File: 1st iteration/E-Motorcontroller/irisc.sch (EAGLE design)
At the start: 173 parts, among them IC1 L298, IC2 L298, U1 KXTJ3-1057, U11 LTC6655CHMS8-3.3PBF, U4 PCA9685, U5 ANALOG_DEVICES_ADXRS646BBGZAN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, U6 ANALOG_DEVICES_AD7997BRUZ-1RE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, U7 MELEXIS_TECHNOLOGIES_MLX90393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, U8 ANALOG_DEVICES_AD7997BRUZ-1RE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, X1 RASPI_BOARD_B+_E4, Y1 16MHz

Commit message: Removed unnecessary stuff in Elrick's 1st iteration PCB's
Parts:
- removed BUCKCONVERTER1: (no value), SO-8:BUCK-CONVERTER5V4A
- removed BUCK_CONVERTER3: LM2695MH, LM2695MH:LM2695MH
- removed C39: 0.1 uF, Wurth_Elektronik_Passive_Capacitors_rev18b:WCAP-CSGP_0805_885012006082_REFLOW
- removed C40: 3 uF, Wurth_Elektronik_Passive_Capacitors_rev18b:WCAP-CSGP_0805_885012006082_REFLOW
- removed C41: 492 nF, Wurth_Elektronik_Passive_Capacitors_rev18b:WCAP-CSGP_0805_885012006018_WAVE
- removed C42, C51: 1 uF, Wurth_Elektronik_Passive_Capacitors_rev18b:WCAP-CSGP_0805_885012006018_WAVE
- removed C43: 22 pF, Wurth_Elektronik_Passive_Capacitors_rev18b:WCAP-CSGP_0805_885012006018_WAVE
- removed C44, C62, C63: 4 uF, Wurth_Elektronik_Passive_Capacitors_rev18b:WCAP-CSGP_0805_885012006018_WAVE
- removed C45: 10 uF, Wurth_Elektronik_Passive_Capacitors_rev18b:WCAP-CSGP_0805_885012006018_WAVE
- removed C46: 22pF, Wurth_Elektronik_Passive_Capacitors_rev18b:WCAP-CSGP_0805_885012006018_WAVE
- removed C47: 47 uF, Wurth_Elektronik_Passive_Capacitors_rev18b:WCAP-CSGP_0805_885012006018_WAVE
- removed C48, C59, C60: 220 uF, Wurth_Elektronik_Passive_Capacitors_rev18b:WCAP-CSGP_0805_885012006018_WAVE
- removed C49: 44 pF, Wurth_Elektronik_Passive_Capacitors_rev18b:WCAP-CSGP_0805_885012006018_WAVE
- removed C50: 2.2 uF, Wurth_Elektronik_Passive_Capacitors_rev18b:WCAP-CSGP_0805_885012006018_WAVE
- removed C52: 100 nF, Wurth_Elektronik_Passive_Capacitors_rev18b:WCAP-CSGP_0805_885012006018_WAVE
- removed C53, C57, C58: 32 uF, Wurth_Elektronik_Passive_Capacitors_rev18b:WCAP-CSGP_0805_885012006018_WAVE
- removed C54: 1.44 pF, Wurth_Elektronik_Passive_Capacitors_rev18b:WCAP-CSGP_0805_885012006018_WAVE
- removed C55: 850 pF, Wurth_Elektronik_Passive_Capacitors_rev18b:WCAP-CSGP_0805_885012006018_WAVE
- removed C56: 3 uF, Wurth_Elektronik_Passive_Capacitors_rev18b:WCAP-CSGP_0805_885012006018_WAVE
- removed C61: 0.1 uF, Wurth_Elektronik_Passive_Capacitors_rev18b:WCAP-CSGP_0805_885012006018_WAVE
- removed D3: 0.75, BeagleBone_Blue_R3:DIODE
- removed FB1, FB2, FB3, FB4: 30Ω/1.8A, SparkFun-Coils:FERRITE_BEAD-0603
- removed J1: (no value), Wurth_Elektronik_Electromechanic_Coaxial _Connectors_rev18a:60314202124525
- removed L7: 24 uH, BeagleBone_Blue_R3:INDUCTOR
- removed L8: 68 uH, BeagleBone_Blue_R3:INDUCTOR
- removed L9: 22uH, BeagleBone_Blue_R3:INDUCTOR
- removed R14: 2k2, SparkFun-Resistors:0.11OHM-2010-1/2W-1%
- removed R15: 3k3, SparkFun-Resistors:0.11OHM-2010-1/2W-1%
- removed R16, R18, R19, R20, R22, R24, R26, R28, R30, R32, R34, R38: 100k, SparkFun-Resistors:100KOHM-0603-1/10W-1%
- removed R17, R21, R23, R25, R27, R29, R31, R33, R35, R37: 10k, SparkFun-Resistors:100KOHM-0603-1/10W-1%
- removed R36: 5.6k, SparkFun-Resistors:5.6KOHM-0603-1/10W-1%
- removed R52: 470 k, adafruit:FLIPFLOP-RES
- removed R53: 47 k, adafruit:FLIPFLOP-RES
- removed R54: 12 k, adafruit:FLIPFLOP-RES
- removed R55, R56, R58: 1 M, adafruit:FLIPFLOP-RES
- removed R57: 200 k, adafruit:FLIPFLOP-RES
- removed R59: 442 k, adafruit:FLIPFLOP-RES
- removed R60: 56 k, adafruit:FLIPFLOP-RES
- removed R61, R64: 10 k, adafruit:FLIPFLOP-RES
- removed R62: 270 k, adafruit:FLIPFLOP-RES
- removed R63: 27 k, adafruit:FLIPFLOP-RES
- removed SELF-TEST, TEMPA@1, TEMPA@2, TEMPA@3, TEMPA@4, TEMPA@5, TEMPA@6, TEMPA@7, TEMPA@8, TEMPA@9: (no value), con-amp-mt:L02P
- removed T1, T2, T3, T4, T5, T6, T7, T8, T9: (no value), DC_LOAD_AU:-PNP-SOT23-BEC
- removed T10: (no value), DC_LOAD_AU:-NPN-SOT23-BEC
- removed TEMPS@1, TEMPS@10, TEMPS@11, TEMPS@12, TEMPS@13, TEMPS@14, TEMPS@15, TEMPS@16, TEMPS@2, TEMPS@3, TEMPS@4, TEMPS@5, TEMPS@6, TEMPS@7, TEMPS@8, TEMPS@9: (no value), con-amp-mt:L03P
- removed U$10: (no value), Analog Devices - AD7997BRUZ-1REEL:AD7175
- removed U$11, U$13, U$15, U$16, U$25, U$26, U$35: 100nF, Nordic_nRF:CAPACITOR_0603_N
- removed U$12, U$42, U$45: 10uF, Nordic_nRF:CAPACITOR_0603_N
- removed U$14, U$19, U$22, U$23, U$24, U$30, U$37, U$38, U$43, U$44, U$46, U$48: 0.1uF, Nordic_nRF:CAPACITOR_0603_N
- removed U$17, U$18: TBD, Nordic_nRF:CAPACITOR_0603_N
- removed U$20, U$31, U$47, U$49, U$7, U$71, U$8, U$9: 1uF, Nordic_nRF:CAPACITOR_0603_N
- removed U$21: 4.7uF, Nordic_nRF:CAPACITOR_0603_N
- removed U$33, U$34: 22nF, Nordic_nRF:CAPACITOR_0603_N
- removed U$36: 10nF, Nordic_nRF:CAPACITOR_0603_N
- removed U$6: NEO-M8, ubloxLib:NEO-M8
- removed U$70: PCF8575C, pcf8575c:PCF8575C
- removed U1: KXTJ3-1057, KXTJ3-1057:KXTJ3-1057
- removed U11: LTC6655CHMS8-3.3PBF, LTC6655CHMS8-3.3PBF:LTC6655CHMS8-3.3PBF
- removed U20: (no value), SOP65P640X120-17N:BUCK_CONVERTER1
- removed U5: ANALOG_DEVICES_ADXRS646BBGZANALOG_DEVICES_ADXRS646BBGZ_0_0, Analog Devices - ADXRS646BBGZ:ANALOG_DEVICES_ADXRS646BBGZANALOG_DEVICES_ADXRS646BBGZ_0_0
- removed U6, U8: ANALOG_DEVICES_AD7997BRUZ-1REELANALOG_DEVICES_AD7997BRUZ-1R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, Analog Devices - AD7997BRUZ-1REEL:ANALOG_DEVICES_AD7997BRUZ-1REELANALOG_DEVICES_AD7997BRUZ-1REEL_0_0
- removed U7: MELEXIS_TECHNOLOGIES_MLX90393SLW-ABA-011-REMELEXIS_TECHNOLO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, Melexis Technologies - MLX90393SLW-ABA-011-RE:MELEXIS_TECHNOLOGIES_MLX90393SLW-ABA-011-REMELEXIS_TECHNOLOGIES_MLX90393S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
- removed X1: RASPI_BOARD_B+_E4, raspberrypi_bastelstube_v13:RASPI_BOARD_B+_E4
- removed Y1: 16MHz, SparkFun-Clocks:CRYSTAL-26MHZSMD-3.2X2.5
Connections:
- removed net 3.3V: C48.2, C49.2, C51.2, C59.2, C60.2, L8.2, R58.2, R64.1, U$6.23_VCC, U$7.2, U$70.A0, U$70.A1, U$70.A2, U$70.VDD, U$71.1, U$8.1, U$9.1, U1.IO_VDD, U1.VDD, U20.BIAS, U7.SENB/CS, U7.VDD, U7.VDD_IO
- removed net ACC-INT: U1.INT, X1.GPIO17
- removed net AGND: FB4.1, R18.1, R19.1, TEMPS@1-1.S, TEMPS@10-1.S, TEMPS@11-1.S, TEMPS@12-1.S, TEMPS@13-1.S, TEMPS@14-1.S, TEMPS@15-1.S, TEMPS@16-1.S, TEMPS@2-1.S, TEMPS@3-1.S, TEMPS@4-1.S, TEMPS@5-1.S, TEMPS@6-1.S, TEMPS@7-1.S, TEMPS@8-1.S, TEMPS@9-1.S, U$37.2, U$42.2, U$43.2, U$44.2, U$45.2, U$46.2, U$47.2, U$48.2, U$49.2, U6.1_AGND, U6.2_AGND, U6.3_AGND, U6.4_AGND, U8.1_AGND, U8.2_AGND, U8.3_AGND, U8.4_AGND, U8.AS
- removed net BUCK-PG: X1.GPIO23
- removed net CE0: U$6.18_SDA/SPI_CS_N, X1.SPI_CE0
- removed net CE4: X1.GPIO24
- removed net CE5: X1.GPIO25
- removed net CE6: X1.GPIO04
- removed net COMP-INT: U7.INT, X1.GPIO27
- removed net COMP-INT-TRIG: U7.INT/TRIG, X1.GPIO22
- removed net GND: BUCKCONVERTER1.GND, FB2.1, U$10.AVSS, U$10.REF-, U$11.2, U$12.2, U$13.2, U$14.2, U$15.2, U$19.2, U$20.2, U$21.2, U$22.2, U$23.1, U$24.1, U$26.2, U$35.2, U11.GND, U11.GND_2, U11.GND_3, U11.GND_4, U5B.1_AGND, U5B.2_AGND
- removed net GPS-INT: U$6.4_EXTINT, X1.GPIO13
- removed net GPS-LNA: U$6.14_LNA_EN/RESERVED, X1.GPIO19
- removed net GPS-RESET: U$6.8_RESET_N, X1.GPIO12
- removed net IO-INT: U$70.!INT, X1.GPIO18
- removed net MOSI: U$10.DIN, U$6.21_RXD/SPI_MOSI, X1.SPI_MOSI
- removed net N$123: BUCK_CONVERTER3.RTN, R53.1, R54.2
- removed net N$124: BUCK_CONVERTER3.VCC, C42.2
- removed net N$125: BUCK_CONVERTER3.BST, C43.2
- removed net N$126: BUCK_CONVERTER3.SW, C43.1, D3.C, L7.1
- removed net N$127: BUCK_CONVERTER3.RON/SD, R52.1
- removed net N$128: BUCK_CONVERTER3.SS, C41.2
- removed net N$129: BUCK_CONVERTER3.ISEN, D3.A
- removed net N$130: R55.1, R56.2, U20.EN
- removed net N$131: C46.2, U20.SS/TRK
- removed net N$132: C47.2, L8.1, U20.SW1, U20.SW2
- removed net N$133: C47.1, U20.CBOOT
- removed net N$134: C49.1, R58.1, R59.2, U20.FB
- removed net N$135: C50.2, U20.VCC
- removed net N$136: BUCKCONVERTER1.LX, C52.1, L9.1
- removed net N$137: BUCKCONVERTER1.FSW, R62.1
- removed net N$138: BUCKCONVERTER1.COMP, C54.2
- removed net N$139: BUCKCONVERTER1.BST, C52.2
- removed net N$140: BUCKCONVERTER1.FB, R60.2, R61.1
- removed net N$141: C54.1, R63.1
- removed net N$142: R64.2, U20.PGOOD
- removed net N$143: R57.2, U20.RT
- removed net N$39: J1.1, U$6.11_RF_IN
- removed net N$40: U$10.XTAL1, U$17.1, Y1.1
- removed net N$42: SELF-TEST-1.S, U5A.1_ST1, U5A.2_ST1
- removed net N$43: R38.2, T10.C
- removed net N$44: U$10.XTAL2, U$18.2, Y1.2
- removed net N$45: U$10.REGCAPA, U$19.1, U$20.1
- removed net N$46: R37.2, T10.B
- removed net N$47: SELF-TEST-2.S, U5A.1_ST2, U5A.2_ST2
- removed net N$48: U$10.REF+, U$12.1, U$13.1, U$14.1, U$21.1, U$22.1, U11.VOUT_F, U11.VOUT_S, U5B.1_VRATIO, U5B.2_VRATIO
- removed net N$50: R14.1, R15.2, U$10.IOVDD
- removed net N$51: U$10.REFCAPD, U$30.1, U$31.1
- removed net N$52: U$35.1, U5A.1_CP5, U5A.2_CP5
- removed net N$53: T10.E, U$36.2, U5A.1_SUMJ, U5A.2_SUMJ
- removed net N$54: U$34.2, U5A.1_CP4, U5A.2_CP4
- removed net N$55: U$34.1, U5A.1_CP3, U5A.2_CP3
- removed net N$56: U$33.2, U5A.1_CP2, U5A.2_CP2
- removed net N$57: U$33.1, U5A.1_CP1, U5A.2_CP1
- removed net N$58: U$10.AIN1, U$36.1, U5A.1_RATEOUT, U5A.2_RATEOUT
- removed net N$59: U$10.AIN0, U5A.1_TEMP, U5A.2_TEMP
- removed net N$60: U$46.1, U$47.1, U8.REFIN
- removed net N$61: U$10.CS
- removed net N$62: R18.2, U8.ALERT/BUSY
- removed net N$63: U$48.1, U$49.1, U6.REFIN
- removed net N$64: U8.!CONVST!
- removed net N$65: R16.1, R17.2, T1.B
- removed net N$66: R37.1, U$10.GPIO0
- removed net N$67: R19.2, U6.ALERT/BUSY
- removed net N$68: U6.!CONVST!
- removed net N$69: T1.C, TEMPA@1-2.S
- removed net N$70: R20.1, R21.2, T2.B
- removed net N$71: T2.C, TEMPA@2-2.S
- removed net N$73: R22.1, R23.2, T3.B
- removed net N$74: T3.C, TEMPA@3-2.S
- removed net N$76: R24.1, R25.2, T4.B
- removed net N$77: T4.C, TEMPA@4-2.S
- removed net N$79: R26.1, R27.2, T5.B
- removed net N$80: T5.C, TEMPA@5-2.S
- removed net N$82: R28.1, R29.2, T6.B
- removed net N$83: T6.C, TEMPA@6-2.S
- removed net N$85: R30.1, R31.2, T7.B
- removed net N$86: T7.C, TEMPA@7-2.S
- removed net N$88: R32.1, R33.2, T8.B
- removed net N$89: T8.C, TEMPA@8-2.S
- removed net N$91: R34.1, R35.2, T9.B
- removed net N$92: T9.C, TEMPA@9-2.S
- removed net SDF: R36.2, U$10.DOUT/RDY
- removed net SS: BUCKCONVERTER1.SS, C55.1
- removed net SYNC: C46.1, R56.1, R57.1, U20.AGND, U20.SYNC
- removed net TEMPA1: R17.1, U$70.P03
- removed net TEMPA2: R21.1, U$70.P04
- removed net TEMPA3: R23.1, U$70.P05
- removed net TEMPA4: R25.1, U$70.P06
- removed net TEMPA5: R27.1, U$70.P07
- removed net TEMPA6: R29.1, U$70.P10
- removed net TEMPA7: R31.1, U$70.P11
- removed net TEMPA8: R33.1, U$70.P12
- removed net TEMPA9: R35.1, U$70.P13
- removed net TEMPS-INT1: U$70.P01
- removed net TEMPS-INT2: U$70.P02
- removed net TEMPS1: TEMPS@1-2.S, U6.VIN1
- removed net TEMPS10: TEMPS@10-2.S, U8.VIN2
- removed net TEMPS11: TEMPS@11-2.S, U8.VIN3
- removed net TEMPS12: TEMPS@12-2.S, U8.VIN4
- removed net TEMPS13: TEMPS@13-2.S, U8.VIN5
- removed net TEMPS14: TEMPS@14-2.S, U8.VIN6
- removed net TEMPS15: TEMPS@15-2.S, U8.VIN7
- removed net TEMPS16: TEMPS@16-2.S, U8.VIN8
- removed net TEMPS2: TEMPS@2-2.S, U6.VIN2
- removed net TEMPS3: TEMPS@3-2.S, U6.VIN3
- removed net TEMPS4: TEMPS@4-2.S, U6.VIN4
- removed net TEMPS5: TEMPS@5-2.S, U6.VIN5
- removed net TEMPS6: TEMPS@6-2.S, U6.VIN6
- removed net TEMPS7: TEMPS@7-2.S, U6.VIN7
- removed net TEMPS8: TEMPS@8-2.S, U6.VIN8
- removed net TEMPS9: TEMPS@9-2.S, U8.VIN1
- removed net VCC: BUCKCONVERTER1.EN, BUCKCONVERTER1.VIN, BUCK_CONVERTER3.VIN, C39.2, C40.2, C45.2, C56.2, C61.2, R52.2, R55.2, U20.VIN1, U20.VIN2
- removed net VCCA: FB1.2, R38.1, U$10.AVDD1, U$10.AVDD2, U$11.1, U$15.1, U$23.2, U$24.2, U$26.1, U11.VIN, U11.~SHDN, U5B.1_AVCC, U5B.2_AVCC
- removed net VCC_1: FB3.2, TEMPS@1-3.S, TEMPS@10-3.S, TEMPS@11-3.S, TEMPS@12-3.S, TEMPS@13-3.S, TEMPS@14-3.S, TEMPS@15-3.S, TEMPS@16-3.S, TEMPS@2-3.S, TEMPS@3-3.S, TEMPS@4-3.S, TEMPS@5-3.S, TEMPS@6-3.S, TEMPS@7-3.S, TEMPS@8-3.S, TEMPS@9-3.S, U$37.1, U$42.1, U$43.1, U$44.1, U$45.1, U6.1_VDD, U6.2_VDD, U6.AS, U8.1_VDD, U8.2_VDD
- net 0: no longer BUCK_CONVERTER3.FB, BUCK_CONVERTER3.SGND, C39.1, C40.1, C41.1, C42.1, C44.1, C45.1, C48.1, C50.1, C51.1, C53.1, C55.2, C56.1, C57.1, C58.1, C59.1, C60.1, C61.1, C62.1, C63.1, FB2.2, FB4.2, J1.2, R15.1, R54.1, R59.1, R61.2, R62.2, R63.2, TEMPA@1-1.S, TEMPA@2-1.S, TEMPA@3-1.S, TEMPA@4-1.S, TEMPA@5-1.S, TEMPA@6-1.S, TEMPA@7-1.S, TEMPA@8-1.S, TEMPA@9-1.S, U$10.DGND, U$16.2, U$17.2, U$18.1, U$25.2, U$30.2, U$31.2, U$38.2, U$6.10_GND, U$6.12_GND, U$6.13_GND, U$6.24_GND, U$6.2_D_SEL, U$7.1, U$70.VSS, U$71.2, U$8.2, U$9.2, U1.ADDR, U1.GND, U1.RES, U20.PGND1, U20.PGND2, U5B.1_PGND, U5B.2_PGND, U7.A0, U7.A1, U7.GND_PAD, U7.VSS, X1.GND, Y1.3
- net 12V: no longer C44.2, C62.2, C63.2, L7.2, R53.2
- net 5V: no longer C53.2, C57.2, C58.2, FB1.1, FB3.1, L9.2, R14.2, R16.2, R20.2, R22.2, R24.2, R26.2, R28.2, R30.2, R32.2, R34.2, R60.1, T1.E, T2.E, T3.E, T4.E, T5.E, T6.E, T7.E, T8.E, T9.E, U$16.1, U$25.1, U$38.1, U5B.1_VDD, U5B.2_VDD, X1.5V0
- net CE1: no longer X1.SPI_CE1
- net CE2: no longer X1.GPIO05
- net CE3: no longer X1.GPIO06
- net CLK: no longer U$10.SCLK, U$6.19_SCL/SPI_CLK, X1.SPI_SCLK
- net MISO: no longer R36.1, U$6.20_TXD/SPI_MISO, X1.SPI_MISO
- net MOTOR-EN1: no longer X1.GPIO16
- net MOTOR-EN2: no longer X1.GPIO26
- net MOTOR-EN3: no longer X1.GPIO20
- net MOTOR-EN4: no longer X1.GPIO21
- net PWM-EN: no longer U$70.P00
- net SCL: no longer U$70.SCL, U1.SCL, U6.SCL, U7.SCL/SCLK, U8.SCL, X1.SCL
- net SDA: no longer U$70.SDA, U1.SDA, U6.SDA, U7.SDA/MOSI, U8.SDA, X1.SDA
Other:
- note removed: "Buck converter: AOZ1284PI"
- note removed: "Buck converter: LM2695MH"
- note removed: "Buck converter: LM43600PWPR"
- note removed: "Gyroscopes"
- note removed: "Power Management"
- note removed: "Sensors and onboard computer"
- note removed: "Thermal Actuators"
- note removed: "Thermal Sensors"

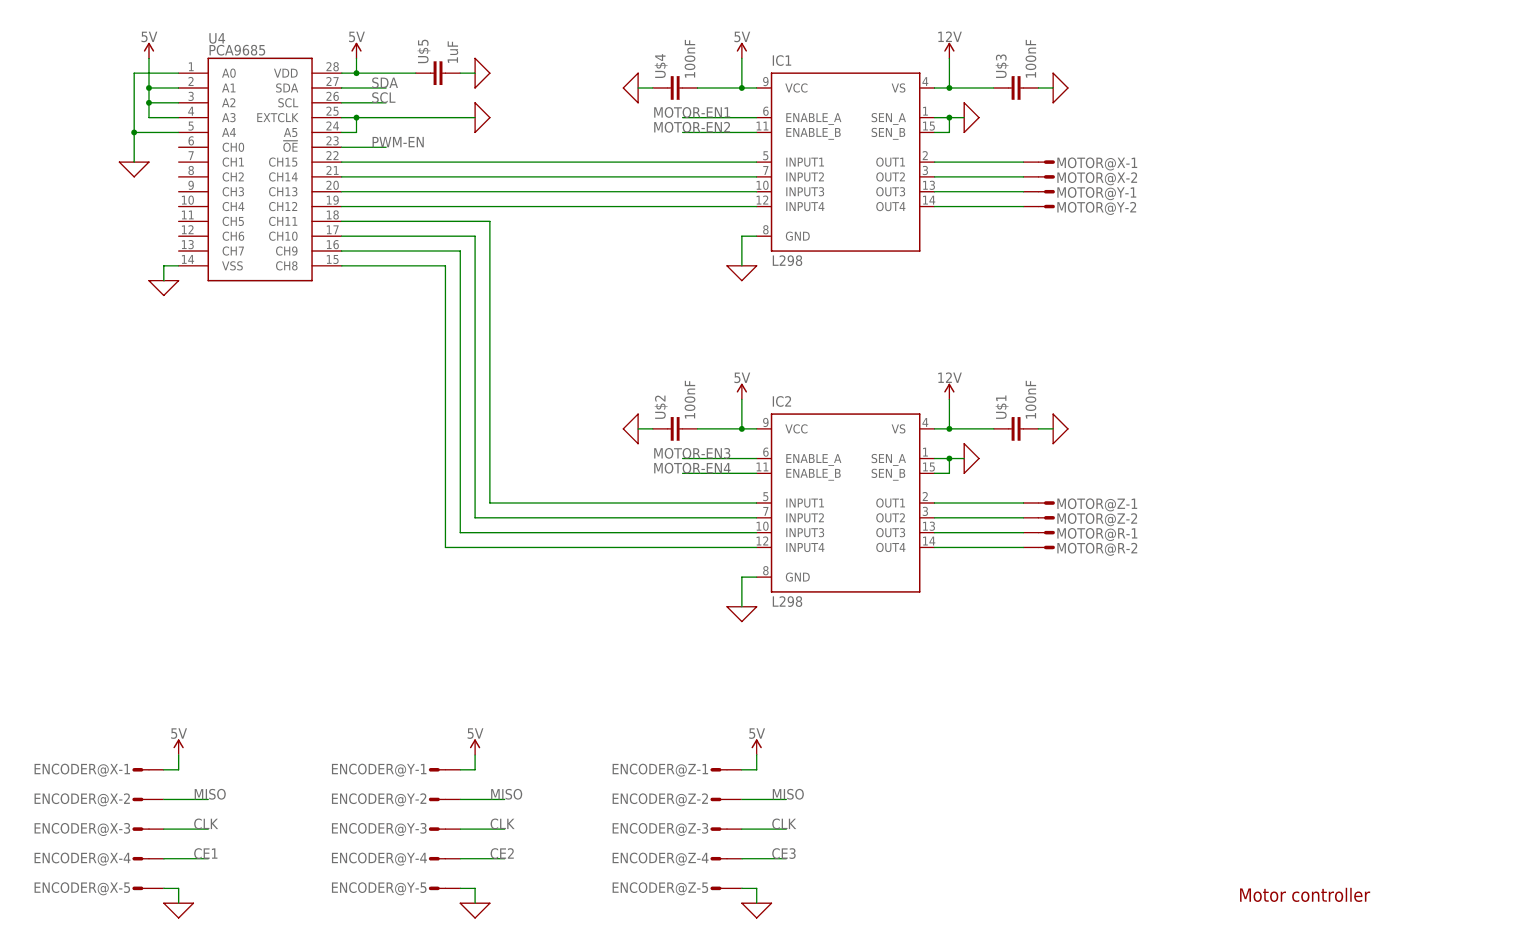
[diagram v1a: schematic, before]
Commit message: 1st iteration update, beginning of the PCB's
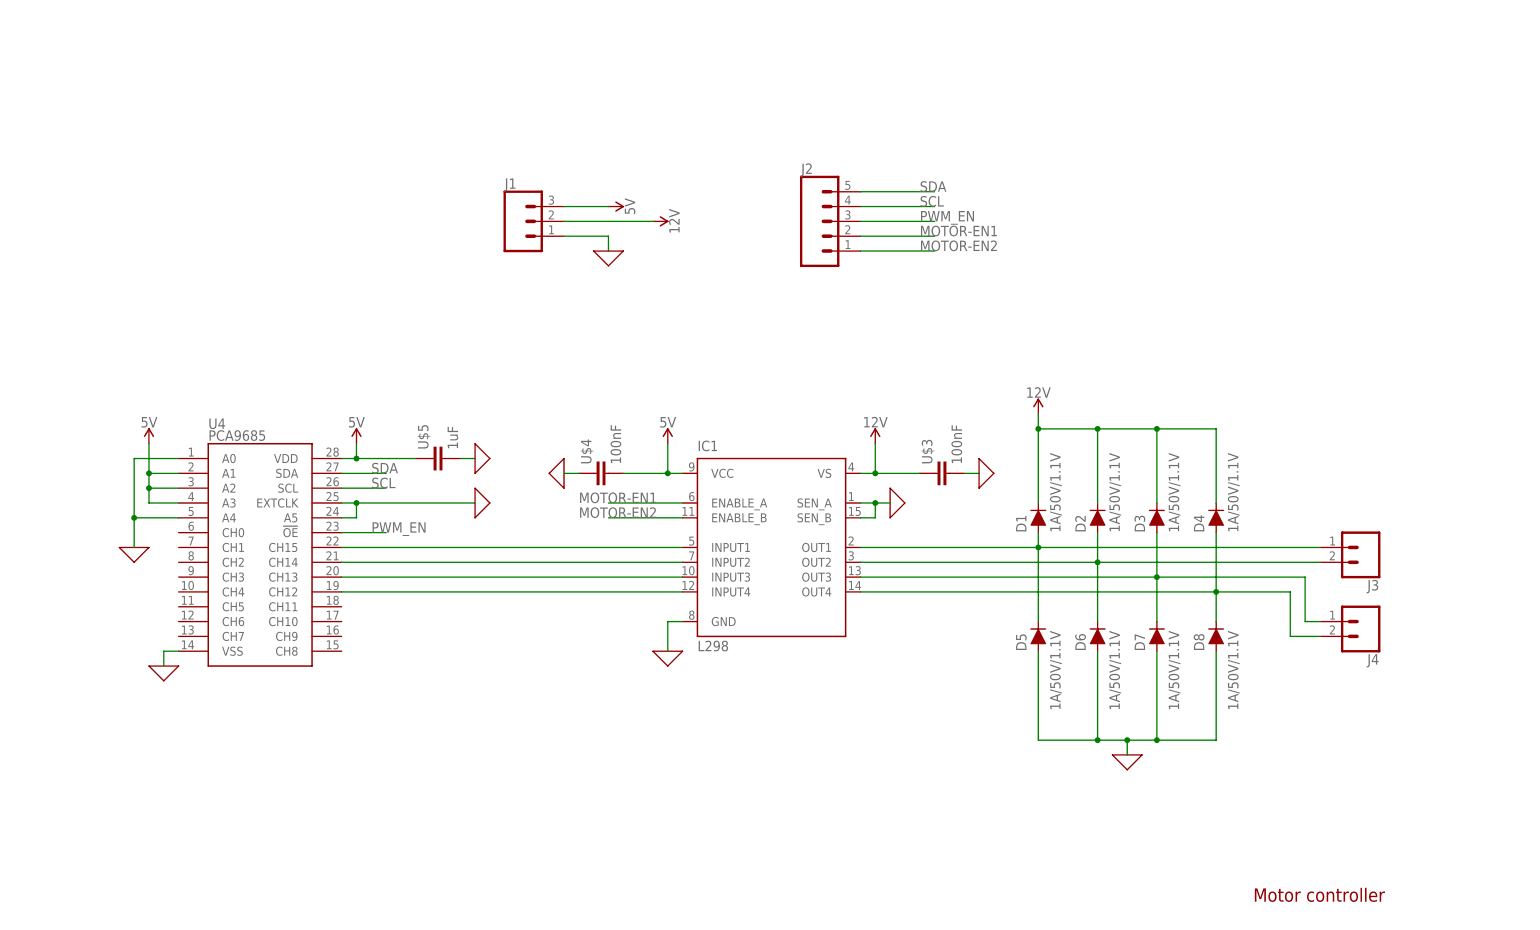
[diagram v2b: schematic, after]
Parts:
- removed ENCODER@X, ENCODER@Y, ENCODER@Z: (no value), con-amp-mt:L05P
- removed IC2: L298, st-microelectronics:L298
- removed MOTOR@R, MOTOR@X, MOTOR@Y, MOTOR@Z: (no value), con-amp-mt:L02P
- removed U$1, U$2: 100nF, Nordic_nRF:CAPACITOR_0805_L
- added D1, D2, D3, D4, D5, D6, D7, D8: 1A/50V/1.1V, SparkFun-DiscreteSemi:DIODE-PTH
- added J1: (no value), SparkFun-Connectors:CONN_03
- added J2: (no value), SparkFun-Connectors:CONN_05
- added J3, J4: (no value), SparkFun-Connectors:CONN_023.5MM
- U$3, U$4: device Nordic_nRF:CAPACITOR_0805_L -> Nordic_nRF:CAPACITOR_0603_L
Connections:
- removed net CE1: ENCODER@X-4.S
- removed net CE2: ENCODER@Y-4.S
- removed net CE3: ENCODER@Z-4.S
- removed net CLK: ENCODER@X-3.S, ENCODER@Y-3.S, ENCODER@Z-3.S
- removed net MISO: ENCODER@X-2.S, ENCODER@Y-2.S, ENCODER@Z-2.S
- removed net MOTOR-EN3: IC2.ENABLE_A
- removed net MOTOR-EN4: IC2.ENABLE_B
- removed net N$22: IC2.INPUT1, U4.CH11
- removed net N$27: IC2.INPUT2, U4.CH10
- removed net N$28: IC2.INPUT3, U4.CH9
- removed net N$30: IC2.INPUT4, U4.CH8
- removed net N$35: IC2.OUT1, MOTOR@Z-1.S
- removed net N$36: IC2.OUT2, MOTOR@Z-2.S
- removed net N$37: IC2.OUT3, MOTOR@R-1.S
- removed net N$38: IC2.OUT4, MOTOR@R-2.S
- removed net PWM-EN: U4.!OE
- new net PWM_EN: J2.3, U4.!OE
- net 0: now also D5.A, D6.A, D7.A, D8.A, J1.1; no longer ENCODER@X-5.S, ENCODER@Y-5.S, ENCODER@Z-5.S, IC2.GND, IC2.SEN_A, IC2.SEN_B, U$1.2, U$2.1
- net 12V: now also D1.C, D2.C, D3.C, D4.C, J1.2; no longer IC2.VS, U$1.1
- net 5V: now also J1.3; no longer ENCODER@X-1.S, ENCODER@Y-1.S, ENCODER@Z-1.S, IC2.VCC, U$2.2
- net MOTOR-EN1: now also J2.2
- net MOTOR-EN2: now also J2.1
- net N$31: now also D1.A, D5.C, J3.1; no longer MOTOR@X-1.S
- net N$32: now also D2.A, D6.C, J3.2; no longer MOTOR@X-2.S
- net N$33: now also D3.A, D7.C, J4.1; no longer MOTOR@Y-1.S
- net N$34: now also D4.A, D8.C, J4.2; no longer MOTOR@Y-2.S
- net SCL: now also J2.4
- net SDA: now also J2.5
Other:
- moved on the sheet: IC1, U$3, U$4, U$5, U4
